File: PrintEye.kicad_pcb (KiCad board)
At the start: 2 copper layers, 18 parts, among them J1 FTDI, J2 Pause Button, J3 Activity LED, Q1 2N7000, Q2 2N7000, U1 ATmega328-PU, Y1 16MHz

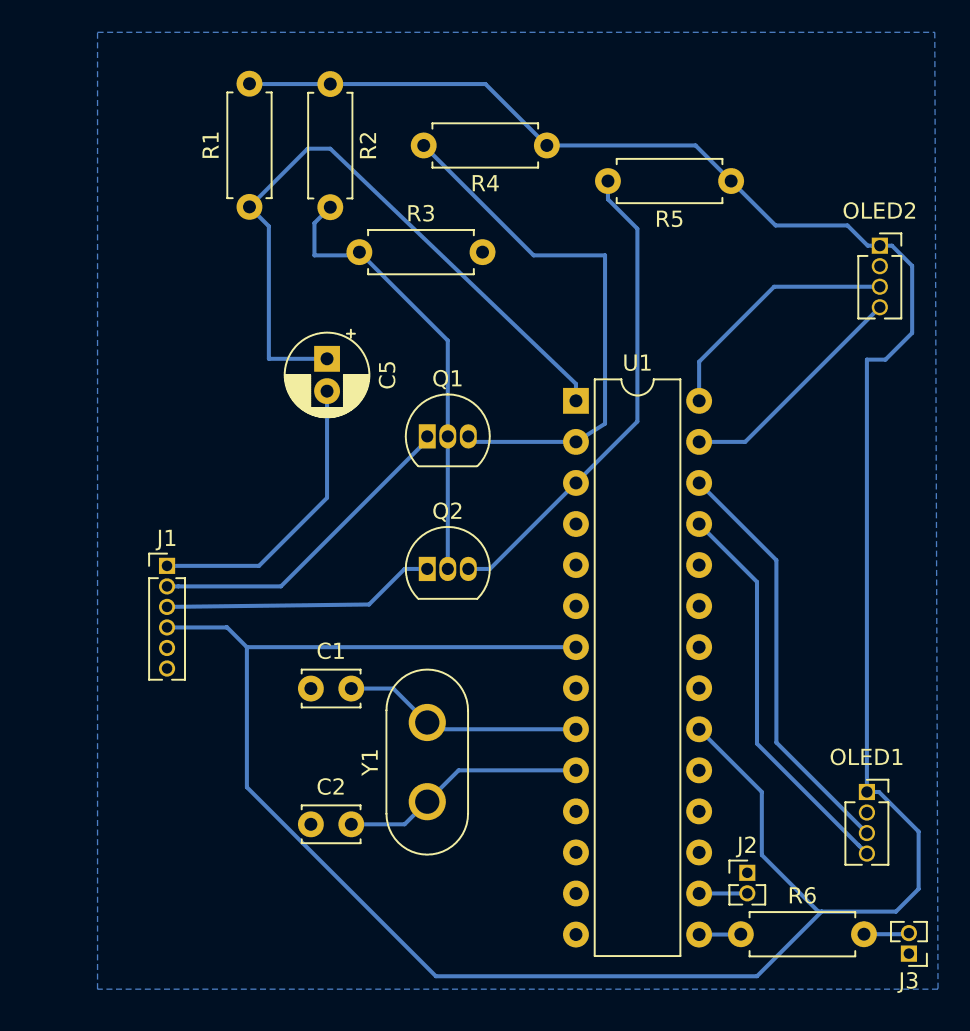
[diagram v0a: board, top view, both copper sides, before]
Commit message: PCB design and footprints
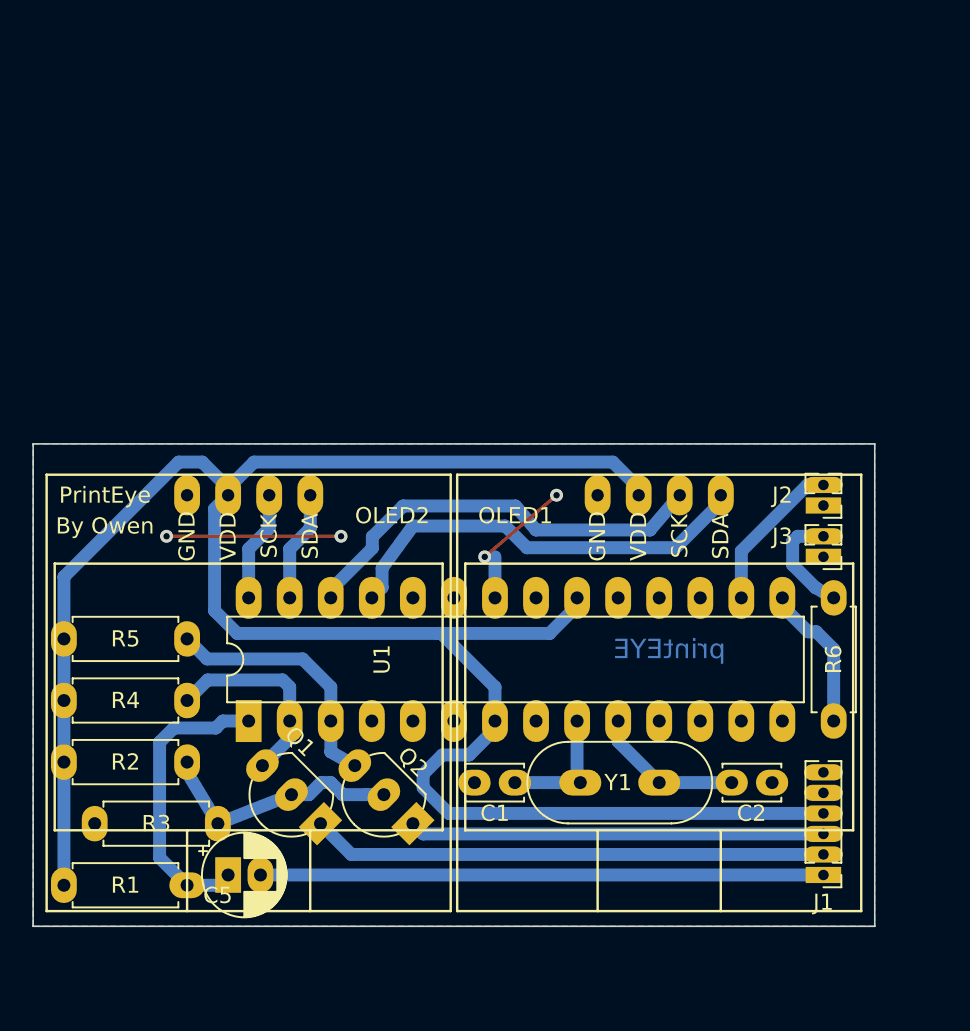
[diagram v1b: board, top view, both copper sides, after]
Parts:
- OLED1, OLED2: value SH1106_I2C_OLED -> SSD1315_I2C_OLED; footprint Connector_PinSocket_1.27mm:PinSocket_1x04_P1.27mm_Vertical -> PrintEyeHardware:SSD1315-I2C-OLED
- Q1, Q2: footprint Package_TO_SOT_THT:TO-92_Inline -> Package_TO_SOT_THT:TO-92_Inline_Wide
- Y1: footprint Crystal:Crystal_HC50_Vertical -> Crystal:Crystal_HC49-4H_Vertical
- moved R5 50.1 mm to (121.9, 100.3), turned to 0 degrees
- moved R4 45.5 mm to (121.9, 104.1), turned to 0 degrees
- moved R2 45.1 mm to (121.9, 108.0), turned to 0 degrees
- moved J1 44.9 mm to (168.9, 114.9), turned to 180 degrees
- moved R1 42.1 mm to (129.5, 115.6), turned to 180 degrees
- moved OLED2 41.5 mm to (133.3, 90.2), turned to 180 degrees
- moved R3 36.4 mm to (131.4, 111.8), turned to 180 degrees
- moved C5 32.5 mm to (132.1, 114.9), turned to 0 degrees
- moved C2 28.7 mm to (165.7, 109.2), turned to 180 degrees
- moved U1 28.3 mm to (133.3, 105.4), turned to 90 degrees
- moved J3 25.1 mm to (168.9, 95.2)
- moved Q1 24.9 mm to (137.8, 111.8), turned to 135 degrees
- moved OLED1 23.5 mm to (158.8, 90.2), turned to 180 degrees
- moved J2 23.2 mm to (168.9, 92.1), turned to 180 degrees
- moved Q2 15.8 mm to (143.5, 111.8), turned to 135 degrees
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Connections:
- net SCL1 renamed SCK1
- net SCL2 renamed SCK2
- J1 pad 5: (no net) -> Net-(J1-Pad5)
- OLED1 pad 1: 5v -> GND
- OLED1 pad 2: GND -> 5v
- OLED2 pad 1: 5v -> GND
- OLED2 pad 2: GND -> 5v
- U1 pad 11: (no net) -> Net-(U1-Pad11)
- U1 pad 12: (no net) -> Net-(U1-Pad12)
- U1 pad 13: (no net) -> Net-(U1-Pad13)
- U1 pad 14: (no net) -> Net-(U1-Pad14)
- U1 pad 17: (no net) -> Net-(U1-Pad17)
- U1 pad 18: (no net) -> Net-(U1-Pad18)
- U1 pad 19: (no net) -> Net-(U1-Pad19)
- U1 pad 21: (no net) -> Net-(U1-Pad21)
- U1 pad 23: (no net) -> Net-(U1-Pad23)
- U1 pad 24: (no net) -> Net-(U1-Pad24)
- U1 pad 4: (no net) -> Net-(U1-Pad4)
- U1 pad 5: (no net) -> Net-(U1-Pad5)
- U1 pad 6: (no net) -> Net-(U1-Pad6)
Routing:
- net 5v: track 185.5 -> 132.0 mm
- net Net-(C5-Pad1): track 42.1 -> 18.4 mm
- net RX: track 33.4 -> 12.6 mm
- net GND: track 0.00 -> 19.2 mm, vias 0 -> 4
- net RTS: track 18.2 -> 34.8 mm
- net TX: track 29.9 -> 15.8 mm
- net 3v3: track 28.1 -> 15.6 mm
- net RX-3v3: track 20.1 -> 31.0 mm
- net SCK2: track 16.2 -> 6.88 mm
- net TX-3v3: track 17.0 -> 25.7 mm
- net SDA2: track 14.6 -> 6.88 mm
- net Net-(C1-Pad2): track 14.9 -> 7.94 mm
- net Net-(J2-Pad2): track 2.98 -> 9.67 mm
- net Net-(R6-Pad1): track 2.59 -> 9.23 mm
- net Net-(C2-Pad2): track 15.3 -> 9.98 mm
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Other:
- board outline added: 52.1 x 29.8 mm
- net class Default: clearance 0.2 -> 0.3; trace_width 0.25 -> 0.8
- rule trace_clearance: 0.2 -> 0.3
- board text added: "By Owen"
- board text added: "PrintEye"
- board text added: "printEYE"
